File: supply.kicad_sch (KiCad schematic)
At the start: 10 parts, among them U2 AP62301WU-7

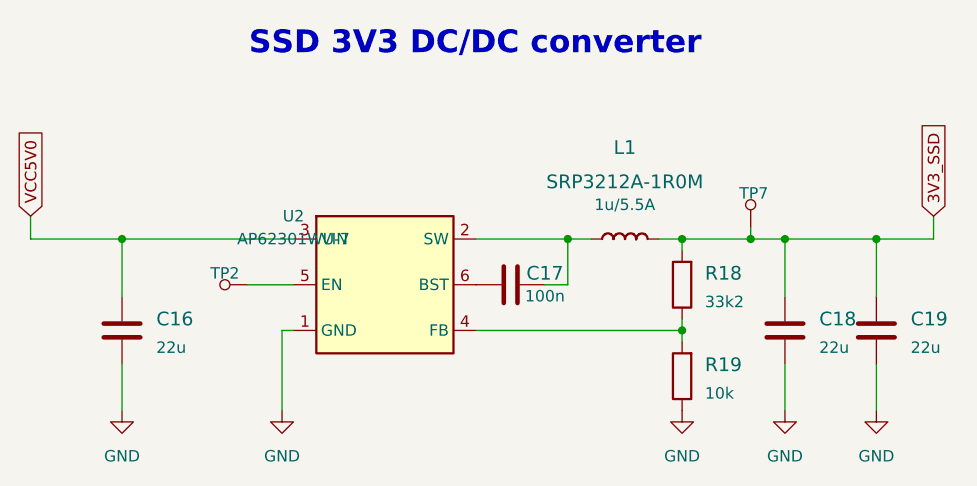
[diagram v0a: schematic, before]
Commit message: Delete copyright field
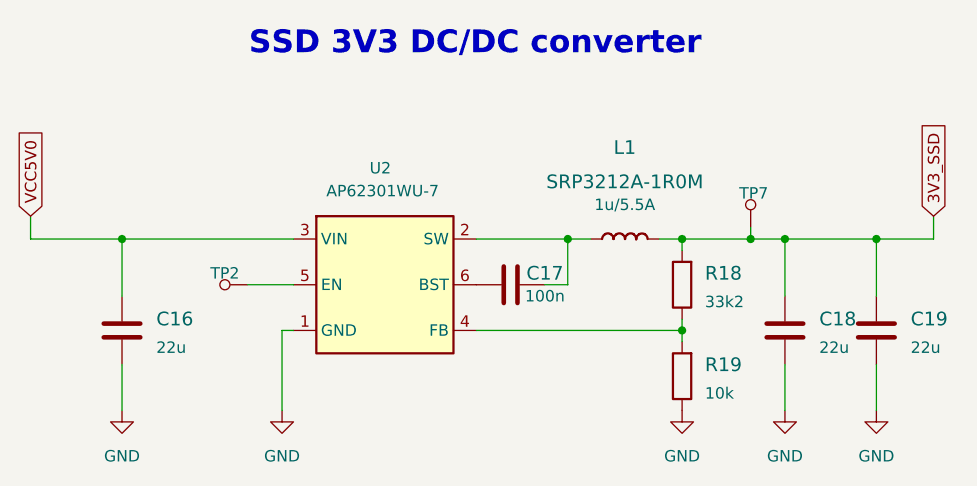
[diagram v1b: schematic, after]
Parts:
- U2: Copyright Copyright (c) 2023 Antmicro -> (none)
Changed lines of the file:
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@@
   )
   (symbol (lib_id "antmicroDCDCConverters:AP62301WU-7") (at 185.42 152.4 0) (unit 1)
-    (in_bom yes) (on_board yes) (fields_autoplaced)
-    (property "Reference" "U2" (id 0) (at 185.42 139.7 0))
-    (property "Value" "AP62301WU-7" (id 1) (at 185.42 142.24 0))
+    (in_bom yes) (on_board yes)
+    (property "Reference" "U2" (id 0) (at 195.072 134.366 0))
+    (property "Value" "AP62301WU-7" (id 1) (at 195.326 136.906 0))
     (property "Footprint" "antmicro-footprints:AP62301WU-7-TSOT23-6" (id 2) (at 220.98 149.86 0)
       (effects (font (size 1.27 1.27) (thickness 0.15)) (justify left bottom) hide)
@@
       (effects (font (size 1.27 1.27) (thickness 0.15)) (justify left bottom) hide)
     )
-    (property "Copyright" "Copyright (c) 2023 Antmicro" (id 8) (at 185.42 152.4 0)
-      (effects (font (size 1.27 1.27)) hide)
-    )
     (pin "1")
